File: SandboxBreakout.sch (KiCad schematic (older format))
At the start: 58 parts

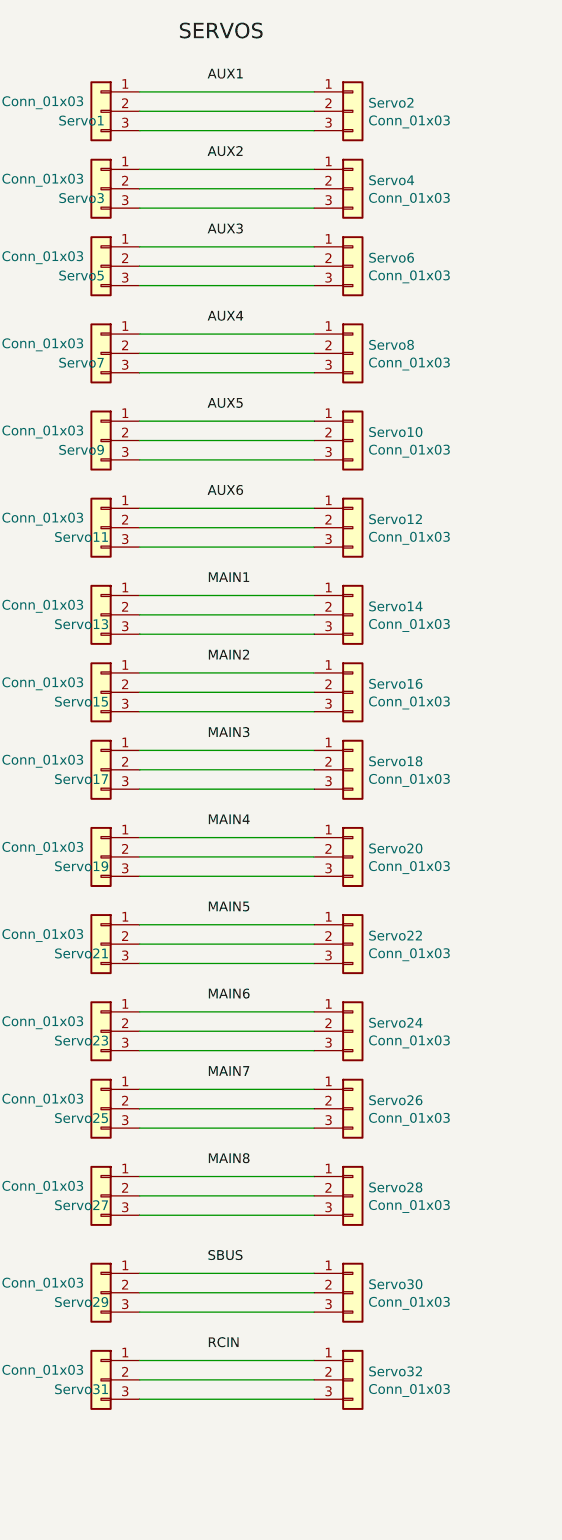
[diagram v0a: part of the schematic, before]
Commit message: Board Draft 1.0
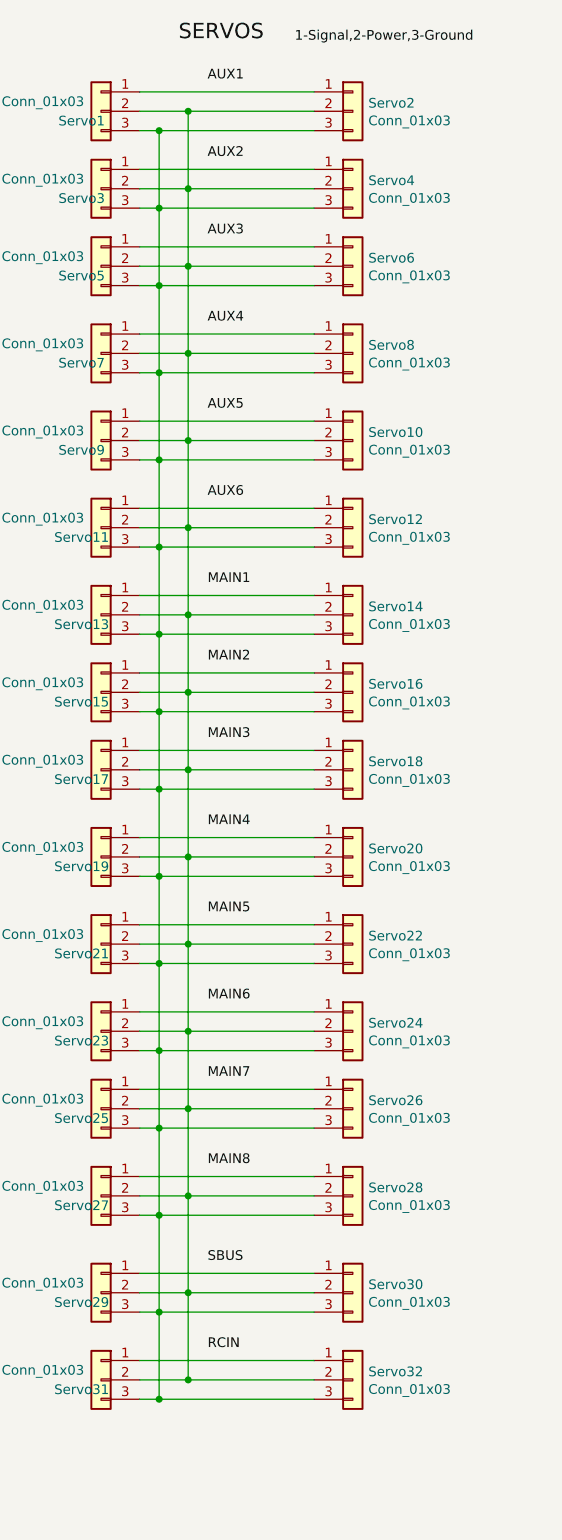
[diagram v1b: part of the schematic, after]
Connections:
- net at Servo1.2 (Pin_2), Servo2.2 (Pin_2): now also Servo10.2 (Pin_2), Servo11.2 (Pin_2), Servo12.2 (Pin_2), Servo13.2 (Pin_2), Servo14.2 (Pin_2), Servo15.2 (Pin_2), Servo16.2 (Pin_2), Servo17.2 (Pin_2), Servo18.2 (Pin_2), Servo19.2 (Pin_2), Servo20.2 (Pin_2), Servo21.2 (Pin_2), Servo22.2 (Pin_2), Servo23.2 (Pin_2), Servo24.2 (Pin_2), Servo25.2 (Pin_2), Servo26.2 (Pin_2), Servo27.2 (Pin_2), Servo28.2 (Pin_2), Servo29.2 (Pin_2), Servo3.2 (Pin_2), Servo30.2 (Pin_2), Servo31.2 (Pin_2), Servo32.2 (Pin_2), Servo4.2 (Pin_2), Servo5.2 (Pin_2), Servo6.2 (Pin_2), Servo7.2 (Pin_2), Servo8.2 (Pin_2), Servo9.2 (Pin_2)
- net at Servo1.3 (Pin_3), Servo2.3 (Pin_3): now also Servo10.3 (Pin_3), Servo11.3 (Pin_3), Servo12.3 (Pin_3), Servo13.3 (Pin_3), Servo14.3 (Pin_3), Servo15.3 (Pin_3), Servo16.3 (Pin_3), Servo17.3 (Pin_3), Servo18.3 (Pin_3), Servo19.3 (Pin_3), Servo20.3 (Pin_3), Servo21.3 (Pin_3), Servo22.3 (Pin_3), Servo23.3 (Pin_3), Servo24.3 (Pin_3), Servo25.3 (Pin_3), Servo26.3 (Pin_3), Servo27.3 (Pin_3), Servo28.3 (Pin_3), Servo29.3 (Pin_3), Servo3.3 (Pin_3), Servo30.3 (Pin_3), Servo31.3 (Pin_3), Servo32.3 (Pin_3), Servo4.3 (Pin_3), Servo5.3 (Pin_3), Servo6.3 (Pin_3), Servo7.3 (Pin_3), Servo8.3 (Pin_3), Servo9.3 (Pin_3)
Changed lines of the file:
@@
 ADC6.6V
 Wire Wire Line
-	2700 2400 3600 2400
-Wire Wire Line
-	2700 1950 3600 1950
-Wire Wire Line
-	2700 1550 3600 1550
+	2700 2400 2800 2400
+Wire Wire Line
+	2700 1950 2800 1950
+Wire Wire Line
+	2700 1550 2800 1550
 $Comp
 L Connector_Generic:Conn_01x03 Servo8
@@
 $EndComp
 Wire Wire Line
-	2700 1150 3600 1150
+	2700 1150 2800 1150
 $Comp
 L Connector_Generic:Conn_01x03 Servo2
@@
 AUX6
 Wire Wire Line
-	2700 3300 3600 3300
-Wire Wire Line
-	2700 2850 3600 2850
+	2700 3300 2800 3300
+Wire Wire Line
+	2700 2850 2800 2850
 $Comp
 L Connector_Generic:Conn_01x03 Servo12
@@
 MAIN4
 Wire Wire Line
-	2700 5000 3600 5000
-Wire Wire Line
-	2700 4550 3600 4550
-Wire Wire Line
-	2700 4150 3600 4150
+	2700 5000 2800 5000
+Wire Wire Line
+	2700 4550 2800 4550
+Wire Wire Line
+	2700 4150 2800 4150
 $Comp
 L Connector_Generic:Conn_01x03 Servo20
@@
 $EndComp
 Wire Wire Line
-	2700 3750 3600 3750
+	2700 3750 2800 3750
 $Comp
 L Connector_Generic:Conn_01x03 Servo14
@@
 MAIN6
 Wire Wire Line
-	2700 5900 3600 5900
-Wire Wire Line
-	2700 5450 3600 5450
+	2700 5900 2800 5900
+Wire Wire Line
+	2700 5450 2800 5450
 $Comp
 L Connector_Generic:Conn_01x03 Servo24
@@
 MAIN8
 Wire Wire Line
-	2700 6750 3600 6750
-Wire Wire Line
-	2700 6300 3600 6300
+	2700 6750 2800 6750
+Wire Wire Line
+	2700 6300 2800 6300
 Wire Wire Line
 	2700 6100 3600 6100
@@
 RCIN
 Wire Wire Line
-	2700 7700 3600 7700
-Wire Wire Line
-	2700 7250 3600 7250
+	2700 7700 2800 7700
+Wire Wire Line
+	2700 7250 2800 7250
 $Comp
 L Connector_Generic:Conn_01x03 Servo32
@@
 	2700 1350 3600 1350
 Wire Wire Line
-	2700 1050 3600 1050
-Wire Wire Line
-	2700 1450 3600 1450
-Wire Wire Line
-	2700 1850 3600 1850
-Wire Wire Line
-	2700 2300 3600 2300
-Wire Wire Line
-	2700 2750 3600 2750
-Wire Wire Line
-	2700 3200 3600 3200
-Wire Wire Line
-	2700 3650 3600 3650
-Wire Wire Line
-	2700 4050 3600 4050
-Wire Wire Line
-	2700 4450 3600 4450
-Wire Wire Line
-	2700 4900 3600 4900
-Wire Wire Line
-	2700 5350 3600 5350
-Wire Wire Line
-	2700 5800 3600 5800
-Wire Wire Line
-	2700 6200 3600 6200
-Wire Wire Line
-	2700 6650 3600 6650
-Wire Wire Line
-	2700 7150 3600 7150
-Wire Wire Line
-	2700 7600 3600 7600
+	2700 2750 2950 2750
+Wire Wire Line
+	2700 3200 2950 3200
+Wire Wire Line
+	2700 3650 2950 3650
+Wire Wire Line
+	2700 4050 2950 4050
+Wire Wire Line
+	2700 4450 2950 4450
+Wire Wire Line
+	2700 4900 2950 4900
+Wire Wire Line
+	2700 5350 2950 5350
+Wire Wire Line
+	2700 5800 2950 5800
+Wire Wire Line
+	2700 6200 2950 6200
+Wire Wire Line
+	2700 6650 2950 6650
+Wire Wire Line
+	2700 7150 2950 7150
+Wire Wire Line
+	2700 7600 2950 7600
+Wire Wire Line
+	2800 1150 2800 1550
+Connection ~ 2800 1150
+Wire Wire Line
+	2800 1150 3600 1150
+Connection ~ 2800 1550
+Wire Wire Line
+	2800 1550 3600 1550
+Wire Wire Line
+	2800 1550 2800 1950
+Connection ~ 2800 1950
+Wire Wire Line
+	2800 1950 3600 1950
+Wire Wire Line
+	2800 2400 2800 1950
+Connection ~ 2800 2400
+Wire Wire Line
+	2800 2400 3600 2400
+Wire Wire Line
+	2800 2400 2800 2850
+Connection ~ 2800 2850
+Wire Wire Line
+	2800 2850 3600 2850
+Wire Wire Line
+	2800 3300 2800 2850
+Connection ~ 2800 3300
+Wire Wire Line
+	2800 3300 3600 3300
+Wire Wire Line
+	2800 3300 2800 3750
+Connection ~ 2800 3750
+Wire Wire Line
+	2800 3750 3600 3750
+Wire Wire Line
+	2800 3750 2800 4150
+Connection ~ 2800 4150
+Wire Wire Line
+	2800 4150 3600 4150
+Wire Wire Line
+	2800 4150 2800 4550
+Connection ~ 2800 4550
+Wire Wire Line
+	2800 4550 3600 4550
+Wire Wire Line
+	2800 4550 2800 5000
+Connection ~ 2800 5000
+Wire Wire Line
+	2800 5000 3600 5000
+Wire Wire Line
+	2800 5000 2800 5450
+Connection ~ 2800 5450
+Wire Wire Line
+	2800 5450 3600 5450
+Wire Wire Line
+	2800 5450 2800 5900
+Connection ~ 2800 5900
+Wire Wire Line
+	2800 5900 3600 5900
+Wire Wire Line
+	2800 5900 2800 6300
+Connection ~ 2800 6300
+Wire Wire Line
+	2800 6300 3600 6300
+Wire Wire Line
+	2800 6300 2800 6750
+Connection ~ 2800 6750
+Wire Wire Line
+	2800 6750 3600 6750
+Wire Wire Line
+	2800 6750 2800 7250
+Connection ~ 2800 7250
+Wire Wire Line
+	2800 7250 3600 7250
+Wire Wire Line
+	2800 7250 2800 7700
+Connection ~ 2800 7700
+Wire Wire Line
+	2800 7700 3600 7700
+Wire Wire Line
+	2950 1050 2950 1450
+Wire Wire Line
+	2700 1050 2950 1050
+Wire Wire Line
+	2950 1050 3600 1050
+Connection ~ 2950 1050
+Wire Wire Line
+	2700 1450 2950 1450
+Wire Wire Line
+	2950 1450 3600 1450
+Connection ~ 2950 1450
+Wire Wire Line
+	2950 1450 2950 1850
+Wire Wire Line
+	2700 1850 2950 1850
+Wire Wire Line
+	2950 1850 3600 1850
+Connection ~ 2950 1850
+Wire Wire Line
+	2950 1850 2950 2300
+Wire Wire Line
+	2700 2300 2950 2300
+Wire Wire Line
+	2950 2300 3600 2300
+Connection ~ 2950 2300
+Wire Wire Line
+	2950 2300 2950 2750
+Connection ~ 2950 2750
+Wire Wire Line
+	2950 2750 3600 2750
+Wire Wire Line
+	2950 2750 2950 3200
+Connection ~ 2950 3200
+Wire Wire Line
+	2950 3200 3600 3200
+Wire Wire Line
+	2950 3200 2950 3650
+Connection ~ 2950 3650
+Wire Wire Line
+	2950 3650 3600 3650
+Wire Wire Line
+	2950 3650 2950 4050
+Connection ~ 2950 4050
+Wire Wire Line
+	2950 4050 3600 4050
+Wire Wire Line
+	2950 4050 2950 4450
+Connection ~ 2950 4450
+Wire Wire Line
+	2950 4450 3600 4450
+Wire Wire Line
+	2950 4450 2950 4900
+Connection ~ 2950 4900
+Wire Wire Line
+	2950 4900 3600 4900
+Wire Wire Line
+	2950 4900 2950 5350
+Connection ~ 2950 5350
+Wire Wire Line
+	2950 5350 3600 5350
+Wire Wire Line
+	2950 5350 2950 5800
+Connection ~ 2950 5800
+Wire Wire Line
+	2950 5800 3600 5800
+Wire Wire Line
+	2950 5800 2950 6200
+Connection ~ 2950 6200
+Wire Wire Line
+	2950 6200 3600 6200
+Wire Wire Line
+	2950 6200 2950 6650
+Connection ~ 2950 6650
+Wire Wire Line
+	2950 6650 3600 6650
+Wire Wire Line
+	2950 6650 2950 7150
+Connection ~ 2950 7150
+Wire Wire Line
+	2950 7150 3600 7150
+Wire Wire Line
+	2950 7150 2950 7600
+Connection ~ 2950 7600
+Wire Wire Line
+	2950 7600 3600 7600
+Text Label 3500 700  0    50   ~ 0
+1-Signal,2-Power,3-Ground
 $EndSCHEMATC
